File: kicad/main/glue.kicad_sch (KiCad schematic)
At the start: 5 parts, among them J8 Conn_01x04_Pin, U5 XC9572XL-10VQG64C

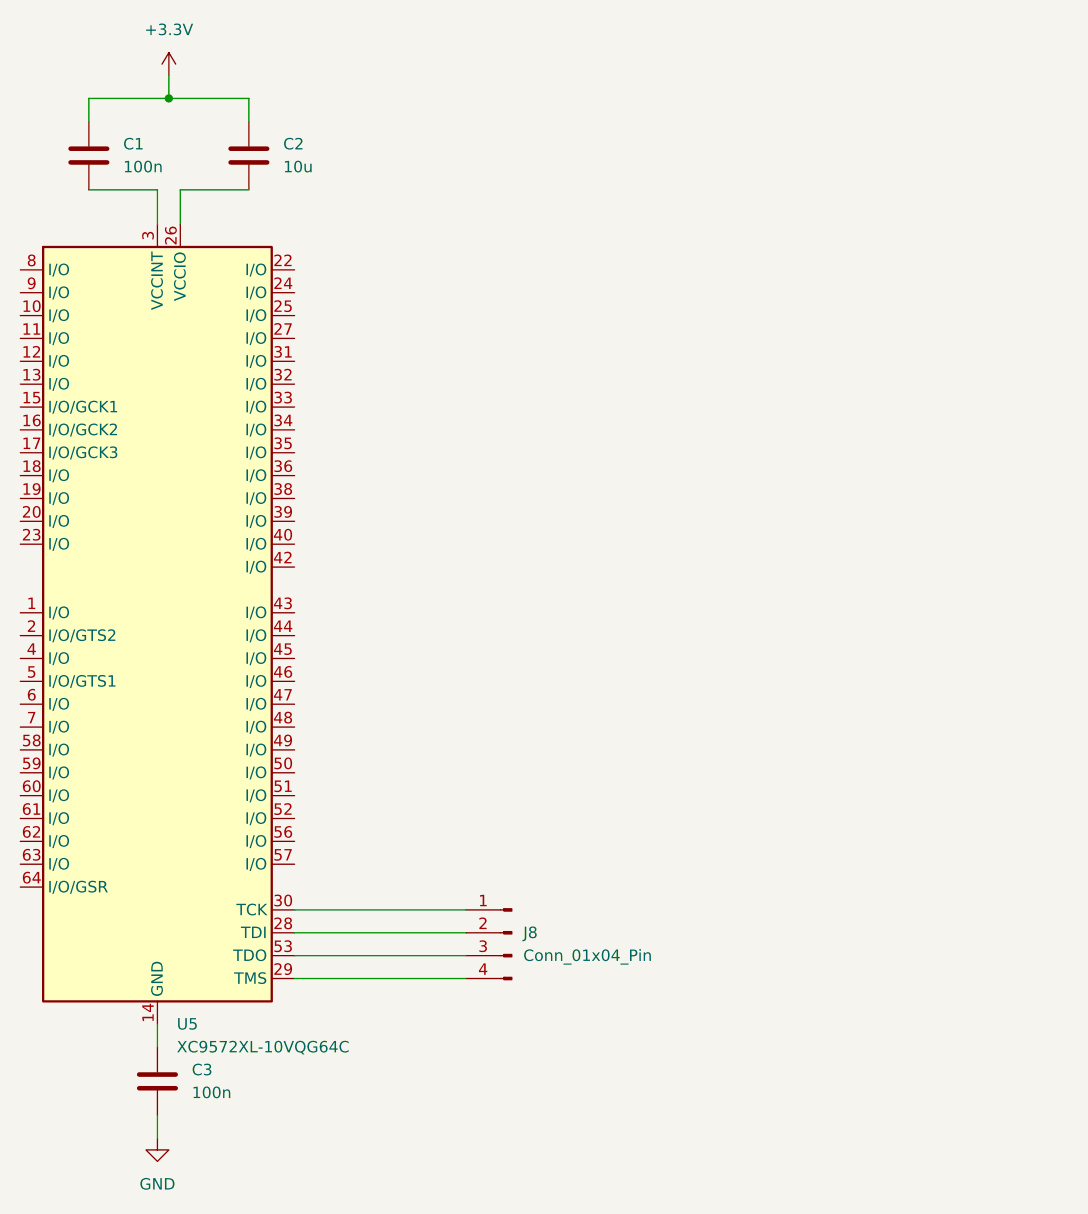
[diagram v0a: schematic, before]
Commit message: fjfjkdsldkjjfds
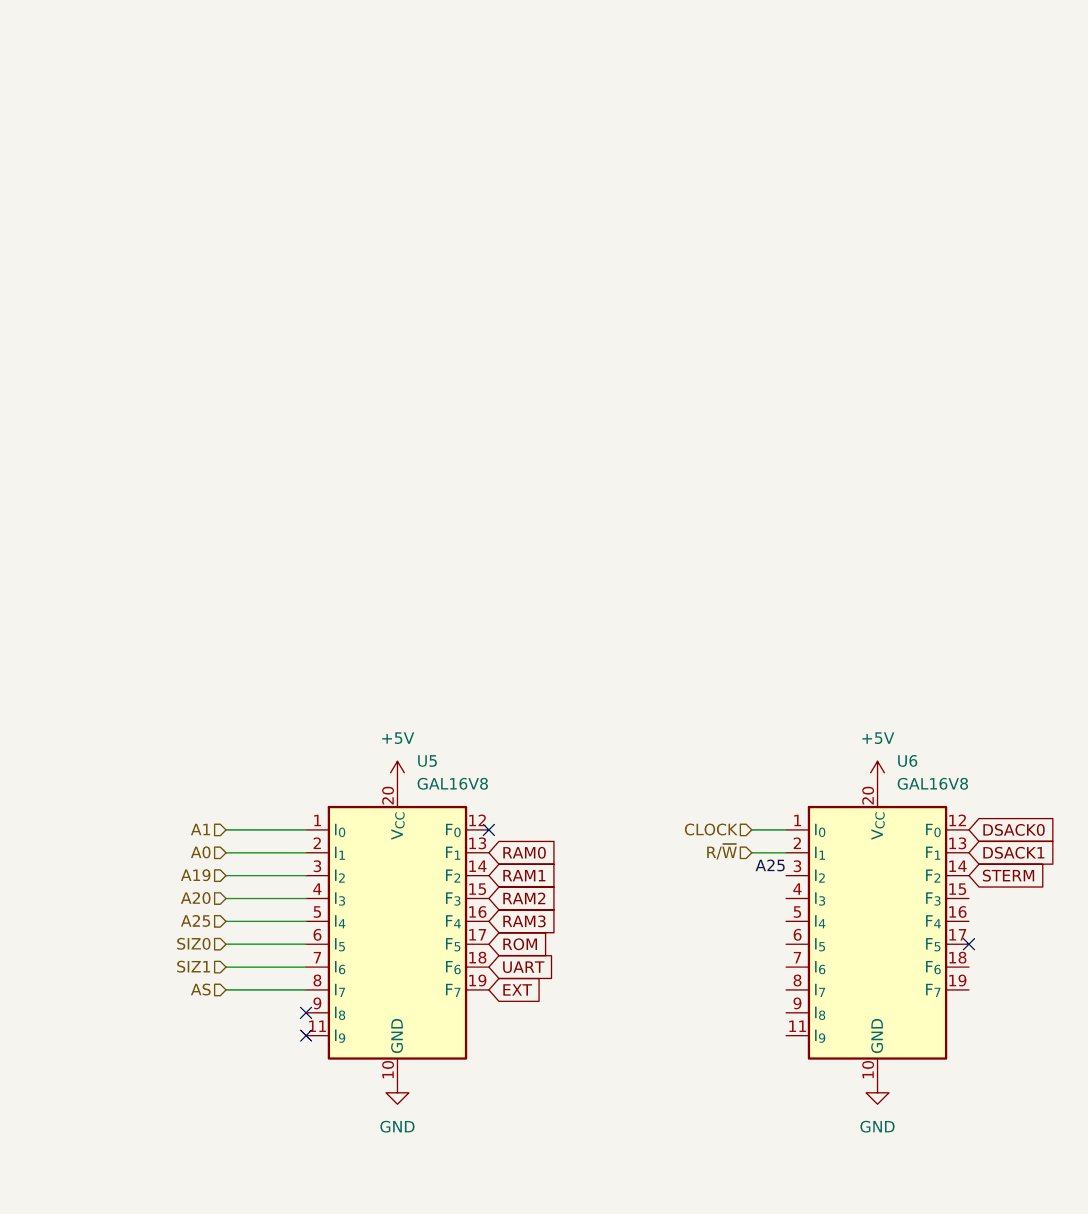
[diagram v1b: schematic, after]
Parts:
- removed C1, C3: 100n, Capacitor_SMD:C_0201_0603Metric, symbol Device:C
- removed C2: 10u, Capacitor_SMD:C_0201_0603Metric, symbol Device:C
- removed J8: Conn_01x04_Pin, Connector_PinHeader_2.54mm:PinHeader_1x04_P2.54mm_Vertical, symbol Connector:Conn_01x04_Pin
- removed U5: XC9572XL-10VQG64C, Package_QFP:TQFP-64_10x10mm_P0.5mm, symbol CPLD_Xilinx:XC9572XL-xxVQx64
- added U5, U6: GAL16V8, Package_DIP:DIP-20_W7.62mm_LongPads, symbol Logic_Programmable:GAL16V8
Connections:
- net GND: now also U5.10 (GND), U6.10 (GND)
- new net +5V: U5.20 (V_{CC}), U6.20 (V_{CC})
- new net A0: U5.2 (I_{1})
- new net A1: U5.1 (I_{0})
- new net A19: U5.3 (I_{2})
- new net A20: U5.4 (I_{3})
- new net A25: U5.5 (I_{4}), U6.3 (I_{2})
- new net AS: U5.8 (I_{7})
- new net CLOCK: U6.1 (I_{0})
- new net DSACK0: U6.12 (F_{0})
- new net DSACK1: U6.13 (F_{1})
- new net EXT: U5.19 (F_{7})
- new net RAM0: U5.13 (F_{1})
- new net RAM1: U5.14 (F_{2})
- new net RAM2: U5.15 (F_{3})
- new net RAM3: U5.16 (F_{4})
- new net ROM: U5.17 (F_{5})
- new net R/~{W}: U6.2 (I_{1})
- new net SIZ0: U5.6 (I_{5})
- new net SIZ1: U5.7 (I_{6})
- new net STERM: U6.14 (F_{2})
- new net UART: U5.18 (F_{6})
- no-connect marks 0 -> 4

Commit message: ygffd
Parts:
- removed U5, U6: GAL16V8, Package_DIP:DIP-20_W7.62mm_LongPads, symbol Logic_Programmable:GAL16V8
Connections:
- no-connect marks 4 -> 0
